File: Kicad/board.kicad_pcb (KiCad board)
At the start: 2 copper layers, 100 x 91.4 mm, 32 parts, among them SW1 SW_Push, SW10 SW_Push, SW11 SW_Push, SW12 SW_Push, SW13 RotaryEncoder, SW2 SW_Push, SW3 SW_Push, SW4 SW_Push, SW5 SW_Push, SW6 SW_Push, SW7 SW_Push, SW8 SW_Push, SW9 SW_Push, U1 XIAO-ESP32-S3-DIP, U2 KY-023, U3 KY-023

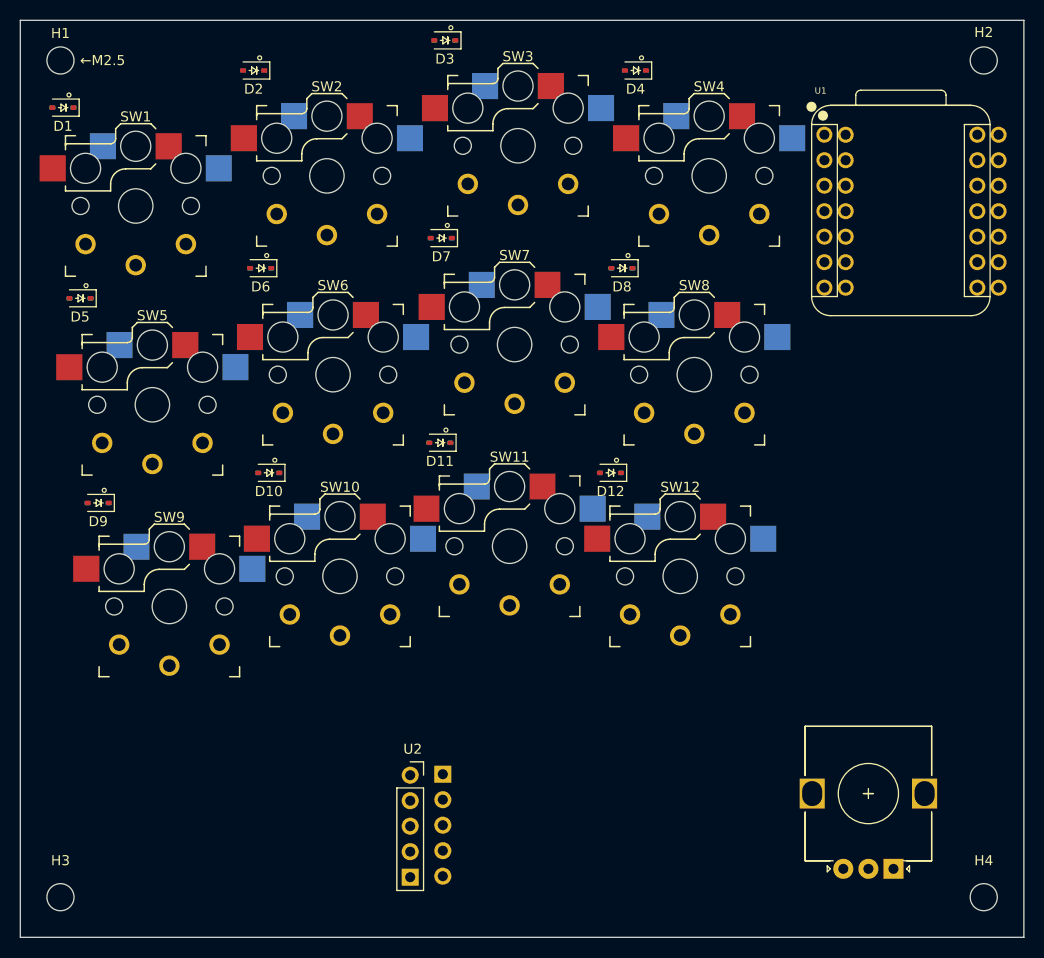
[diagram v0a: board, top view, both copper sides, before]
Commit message: [update] routed
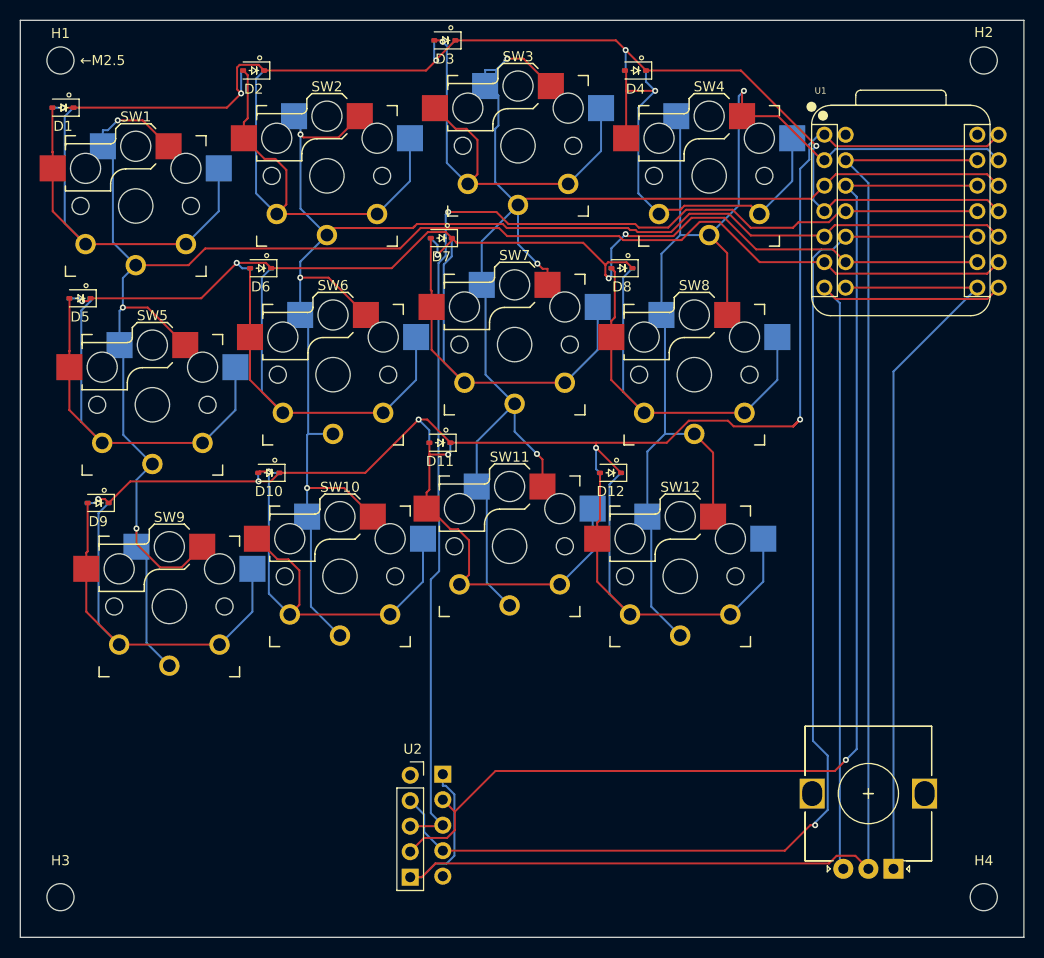
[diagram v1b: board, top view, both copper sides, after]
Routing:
- net column1: track 0.00 -> 175.8 mm, vias 0 -> 3
- net column2: track 0.00 -> 151.8 mm, vias 0 -> 3
- net GNDPWR: track 0.00 -> 145.8 mm
- net row3: track 0.00 -> 139.3 mm, vias 0 -> 5
- net column3: track 0.00 -> 138.5 mm, vias 0 -> 3
- net column4: track 0.00 -> 125.2 mm, vias 0 -> 1
- net VCC: track 0.00 -> 121.2 mm, vias 0 -> 1
- net joystick_x: track 0.00 -> 121.2 mm, vias 0 -> 1
- net joystick_y: track 0.00 -> 119.4 mm, vias 0 -> 1
- net row1: track 0.00 -> 117.7 mm, vias 0 -> 5
- net row2: track 0.00 -> 113.1 mm, vias 0 -> 5
- net rotary_encoder_b: track 0.00 -> 77.0 mm
- net rotary_encoder_a: track 0.00 -> 74.5 mm
- net Net-(D2-A): track 0.00 -> 51.8 mm
- net Net-(D8-A): track 0.00 -> 50.6 mm
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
